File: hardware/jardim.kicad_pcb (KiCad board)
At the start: 2 copper layers, 100 x 100 mm, 90 parts, among them J1 DC_INPUT, J10 DHT22_AMB, J11 LIGHT_SENSOR_1, J12 LIGHT_SENSOR_2, J13 LEVEL_SENSOR_1, J14 LEVEL_SENSOR_2, J15 SOIL_HUMIDITY_SENSOR_1, J16 SOIL_HUMIDITY_SENSOR_2, J18 USB_C_Receptacle_PowerOnly_6P, J2 PUMP_1, J3 PUMP_2, J4 LIGHT_1, J5 LIGHG_2, J6 HEAT_1, J7 HEAT_2, J8 DS12B20_2, J9 DS18B20_1, Q1 FQP30N06L, Q2 FQP30N06L, Q3 FQP30N06L, Q4 FQP30N06L, Q5 FQP30N06L, Q6 FQP30N06L, Q7 BC337, SW1 SW_Push, SW2 SW_Push, SW3 SW_Push, SW4 SW_SPST, U1 AM2302, U2 DM-OLED096-636

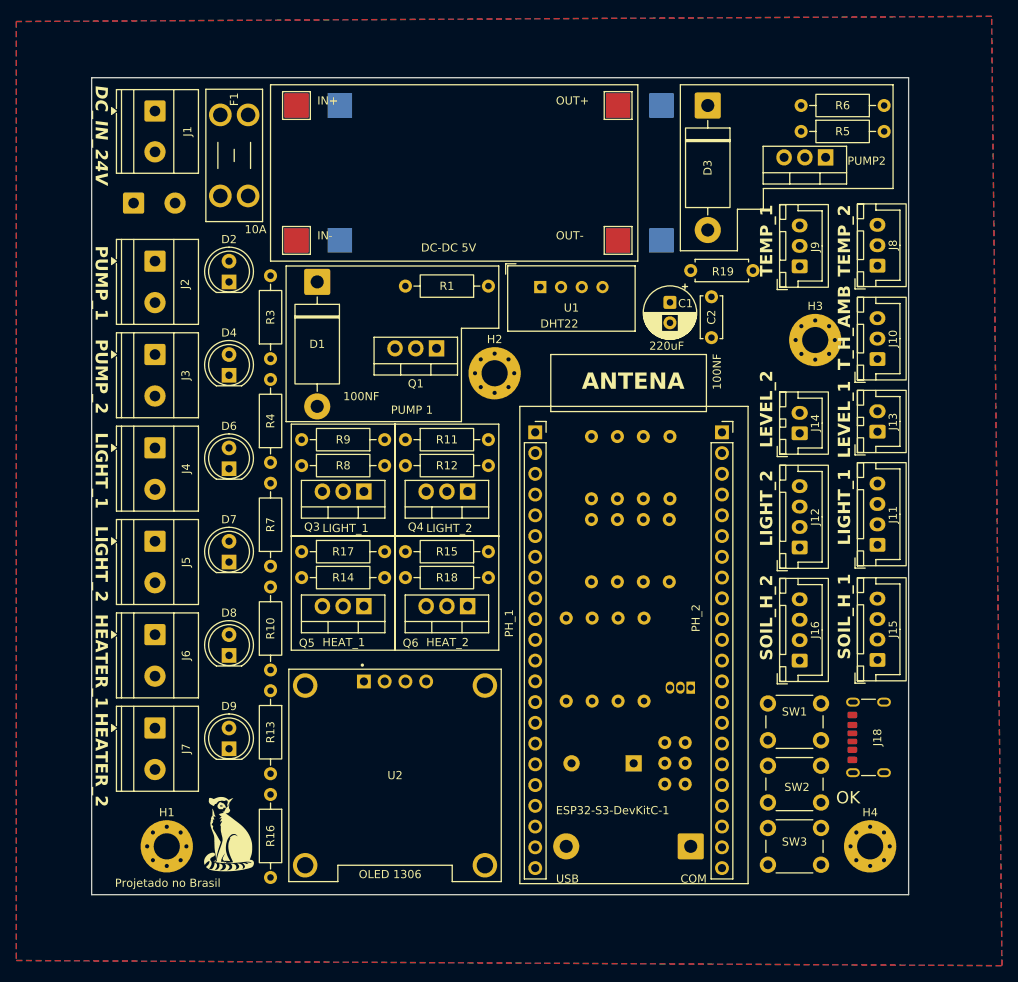
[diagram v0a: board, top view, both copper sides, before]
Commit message: sem avisos, pronto para rotear
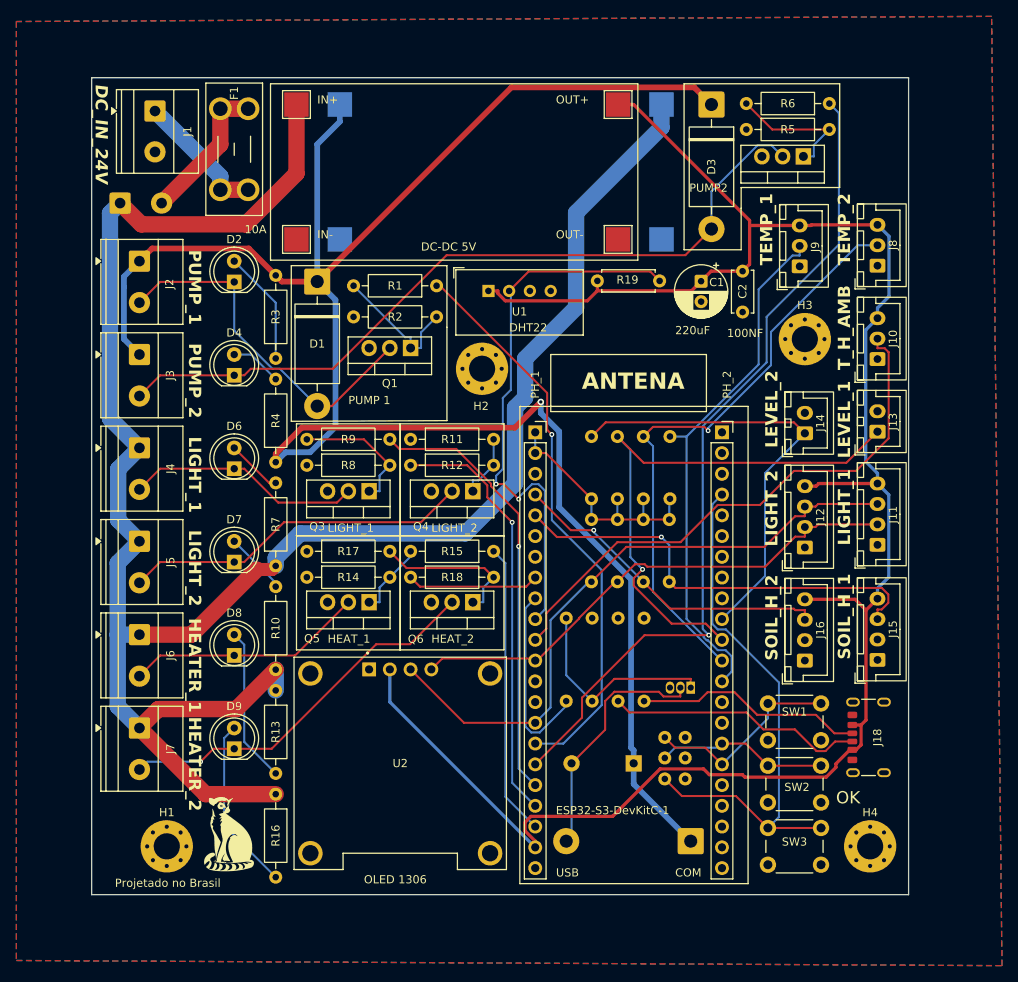
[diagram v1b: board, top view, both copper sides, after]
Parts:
- added R2: 10k, Resistor_THT:R_Axial_DIN0207_L6.3mm_D2.5mm_P10.16mm_Horizontal, F.Cu at (124.5, 67.3)
- moved R19 19.1 mm to (154.3, 62.9), turned to 0 degrees
- moved R5 6.71 mm to (172.5, 44.3)
- moved R6 6.71 mm to (182.7, 41.2)
- moved U1 6.37 mm to (141.0, 64.1)
- moved R1 6.35 mm to (134.6, 63.5)
- moved C2 4.93 mm to (172.1, 61.7)
- moved C1 4.61 mm to (167.0, 62.9)
- moved Q1 3.18 mm to (131.4, 71.1)
- moved Q2 2.72 mm to (179.5, 47.6)
- moved J2 1.91 mm to (98.3, 60.4)
- moved J3 1.91 mm to (98.3, 71.9)
- moved J4 1.91 mm to (98.3, 83.3)
- moved J5 1.91 mm to (98.3, 94.7)
- moved J6 1.91 mm to (98.3, 106.2)
- moved J7 1.91 mm to (98.3, 117.6)
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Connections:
- net Net-(SW4-B) renamed /VIN_AFTER_FUSE
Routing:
- net +24V: track 0.00 -> 257.2 mm
- net +12V: track 0.00 -> 244.2 mm, vias 0 -> 1
- net +5V: track 0.00 -> 243.7 mm
- net /IO11: track 0.00 -> 102.0 mm, vias 0 -> 1
- net /PUMP_2_SW_NEG: track 0.00 -> 94.7 mm
- net /IO9: track 0.00 -> 77.9 mm
- net /IO36: track 0.00 -> 72.7 mm, vias 0 -> 1
- net /IO10: track 0.00 -> 70.0 mm, vias 0 -> 1
- net /IO17: track 0.00 -> 68.5 mm, vias 0 -> 2
- net /IO37: track 0.00 -> 68.3 mm, vias 0 -> 1
- net /IO18: track 0.00 -> 67.9 mm
- net /IO1: track 0.00 -> 67.4 mm
- net /IO35: track 0.00 -> 65.0 mm
- net /IO8: track 0.00 -> 63.7 mm
- net /IO38: track 0.00 -> 54.3 mm
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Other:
- board text removed: "10k"
